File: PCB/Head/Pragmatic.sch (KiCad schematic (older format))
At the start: 11 parts, among them J1 Conn_02x07_Odd_Even, J2 Conn_02x07_Odd_Even, SW1 SW_Push, SW2 SW_Push, SW3 SW_Push, SW4 SW_Push, U1 ProMicro

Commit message: left ready
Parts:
- removed D1, D2, D3, D4: D, Foostan:D3_SMD_v2, symbol Device:D
- removed SW1, SW2, SW3, SW4: SW_Push, Foostan:CherryMX_ChocV2_1u, symbol Switch:SW_Push
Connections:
- wire segments 14 -> 0
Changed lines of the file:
@@
 Comment4 ""
 $EndDescr
-Text GLabel 1400 2100 0    50   Input ~ 0
-Row1
-Text GLabel 1400 2650 0    50   Input ~ 0
-Row2
-Text GLabel 2100 1550 1    50   Input ~ 0
-Col1
-Text GLabel 2600 1550 1    50   Input ~ 0
-Col2
-$Comp
-L Device:D D1
-U 1 1 618785C9
-P 1700 1950
-F 0 "D1" V 1700 1870 50  0000 R CNN
-F 1 "D" H 1700 2076 50  0001 C CNN
-F 2 "Foostan:D3_SMD_v2" H 1700 1950 50  0001 C CNN
-F 3 "~" H 1700 1950 50  0001 C CNN
-	1    1700 1950
-	0    -1   -1   0
-$EndComp
-Wire Wire Line
-	1400 2100 1700 2100
-Wire Wire Line
-	1400 2650 1700 2650
-$Comp
-L Switch:SW_Push SW1
-U 1 1 6187A774
-P 1900 1800
-F 0 "SW1" H 1900 1993 50  0000 C CNN
-F 1 "SW_Push" H 1900 1994 50  0001 C CNN
-F 2 "Foostan:CherryMX_ChocV2_1u" H 1900 2000 50  0001 C CNN
-F 3 "~" H 1900 2000 50  0001 C CNN
-	1    1900 1800
-	1    0    0    -1
-$EndComp
-Connection ~ 1700 2100
-Wire Wire Line
-	1700 2100 2200 2100
-$Comp
-L Device:D D3
-U 1 1 618803D0
-P 1700 2500
-F 0 "D3" V 1700 2420 50  0000 R CNN
-F 1 "D" H 1700 2626 50  0001 C CNN
-F 2 "Foostan:D3_SMD_v2" H 1700 2500 50  0001 C CNN
-F 3 "~" H 1700 2500 50  0001 C CNN
-	1    1700 2500
-	0    -1   -1   0
-$EndComp
-$Comp
-L Switch:SW_Push SW3
-U 1 1 618803DA
-P 1900 2350
-F 0 "SW3" H 1900 2543 50  0000 C CNN
-F 1 "SW_Push" H 1900 2544 50  0001 C CNN
-F 2 "Foostan:CherryMX_ChocV2_1u" H 1900 2550 50  0001 C CNN
-F 3 "~" H 1900 2550 50  0001 C CNN
-	1    1900 2350
-	1    0    0    -1
-$EndComp
-Connection ~ 2100 2350
-Wire Wire Line
-	2100 2350 2100 2650
-Wire Wire Line
-	2100 1550 2100 1800
-Wire Wire Line
-	2100 1800 2100 2350
-Connection ~ 2100 1800
-$Comp
-L Device:D D2
-U 1 1 6188DF74
-P 2200 1950
-F 0 "D2" V 2200 1870 50  0000 R CNN
-F 1 "D" H 2200 2076 50  0001 C CNN
-F 2 "Foostan:D3_SMD_v2" H 2200 1950 50  0001 C CNN
-F 3 "~" H 2200 1950 50  0001 C CNN
-	1    2200 1950
-	0    -1   -1   0
-$EndComp
-$Comp
-L Switch:SW_Push SW2
-U 1 1 6188DF7C
-P 2400 1800
-F 0 "SW2" H 2400 1993 50  0000 C CNN
-F 1 "SW_Push" H 2400 1994 50  0001 C CNN
-F 2 "Foostan:CherryMX_ChocV2_1u" H 2400 2000 50  0001 C CNN
-F 3 "~" H 2400 2000 50  0001 C CNN
-	1    2400 1800
-	1    0    0    -1
-$EndComp
-Connection ~ 2200 2100
-Wire Wire Line
-	2200 2100 2700 2100
-$Comp
-L Device:D D4
-U 1 1 6188DF84
-P 2200 2500
-F 0 "D4" V 2200 2420 50  0000 R CNN
-F 1 "D" H 2200 2626 50  0001 C CNN
-F 2 "Foostan:D3_SMD_v2" H 2200 2500 50  0001 C CNN
-F 3 "~" H 2200 2500 50  0001 C CNN
-	1    2200 2500
-	0    -1   -1   0
-$EndComp
-$Comp
-L Switch:SW_Push SW4
-U 1 1 6188DF8A
-P 2400 2350
-F 0 "SW4" H 2400 2543 50  0000 C CNN
-F 1 "SW_Push" H 2400 2544 50  0001 C CNN
-F 2 "Foostan:CherryMX_ChocV2_1u" H 2400 2550 50  0001 C CNN
-F 3 "~" H 2400 2550 50  0001 C CNN
-	1    2400 2350
-	1    0    0    -1
-$EndComp
-Connection ~ 2600 2350
-Wire Wire Line
-	2600 2350 2600 2650
-Wire Wire Line
-	2600 1550 2600 1800
-Wire Wire Line
-	2600 1800 2600 2350
-Connection ~ 2600 1800
-Wire Wire Line
-	2200 2650 2600 2650
-Connection ~ 1700 2650
-Connection ~ 2200 2650
-Wire Wire Line
-	1700 2650 2100 2650
 Text GLabel 4800 3800 0    50   Input ~ 0
 Row2
@@
 Text GLabel 6200 3600 2    50   Input ~ 0
 VCC
-Text GLabel 6600 3350 3    50   Input ~ 0
-VCC
-$Comp
-L power:+5V #PWR0101
-U 1 1 6186CA9E
-P 6600 3350
-F 0 "#PWR0101" H 6600 3200 50  0001 C CNN
-F 1 "+5V" H 6615 3523 50  0000 C CNN
-F 2 "" H 6600 3350 50  0001 C CNN
-F 3 "" H 6600 3350 50  0001 C CNN
-	1    6600 3350
-	1    0    0    -1
-$EndComp
 Text GLabel 7000 3650 0    50   Input ~ 0
 VCC
@@
 Text GLabel 4100 3650 2    50   Input ~ 0
 Ground
-Text GLabel 4100 3850 2    50   Input ~ 0
+Text GLabel 3600 4050 0    50   Input ~ 0
 Col1
-Text GLabel 4100 3950 2    50   Input ~ 0
+Text GLabel 4100 4050 2    50   Input ~ 0
 Col2
 Text GLabel 4800 3700 0    50   Input ~ 0
@@
 Text GLabel 4800 4100 0    50   Input ~ 0
 Col5
+Text GLabel 4100 4250 2    50   Input ~ 0
+Col6
 Text GLabel 3600 4250 0    50   Input ~ 0
-Col6
-Text GLabel 4100 4250 2    50   Input ~ 0
 Col5
 Text GLabel 4100 4150 2    50   Input ~ 0
@@
 Text GLabel 4800 3900 0    50   Input ~ 0
 Col3
-Text GLabel 4100 4050 2    50   Input ~ 0
+Text GLabel 3600 4150 0    50   Input ~ 0
 Col3
-Text GLabel 3600 4150 0    50   Input ~ 0
+Text GLabel 4100 3850 2    50   Input ~ 0
 Row4
-Text GLabel 3600 4050 0    50   Input ~ 0
+Text GLabel 3600 3950 0    50   Input ~ 0
 Row5
-Text GLabel 3600 3950 0    50   Input ~ 0
+Text GLabel 4100 3950 2    50   Input ~ 0
 Row6
 $Comp
@@
 	1    0    0    -1
 $EndComp
-Connection ~ 2100 2650
-Wire Wire Line
-	2100 2650 2200 2650
-Connection ~ 2600 2650
-Wire Wire Line
-	2600 2650 2700 2650
+$Comp
+L power:+5V #PWR0101
+U 1 1 6186CA9E
+P 6600 3350
+F 0 "#PWR0101" H 6600 3200 50  0001 C CNN
+F 1 "+5V" H 6615 3523 50  0000 C CNN
+F 2 "" H 6600 3350 50  0001 C CNN
+F 3 "" H 6600 3350 50  0001 C CNN
+	1    6600 3350
+	1    0    0    -1
+$EndComp
+Text GLabel 6600 3350 3    50   Input ~ 0
+VCC
 $EndSCHEMATC

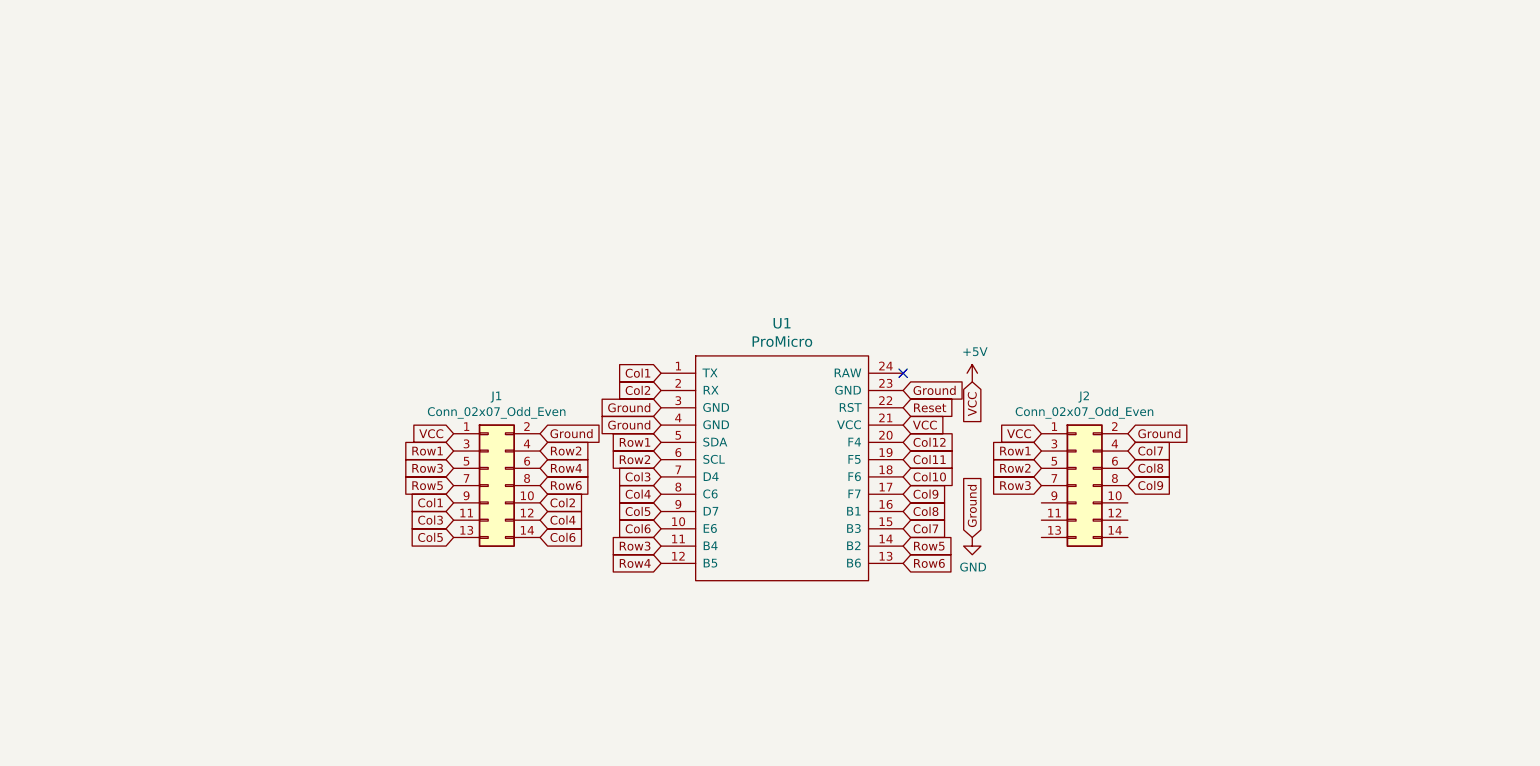
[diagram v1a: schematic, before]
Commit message: head board
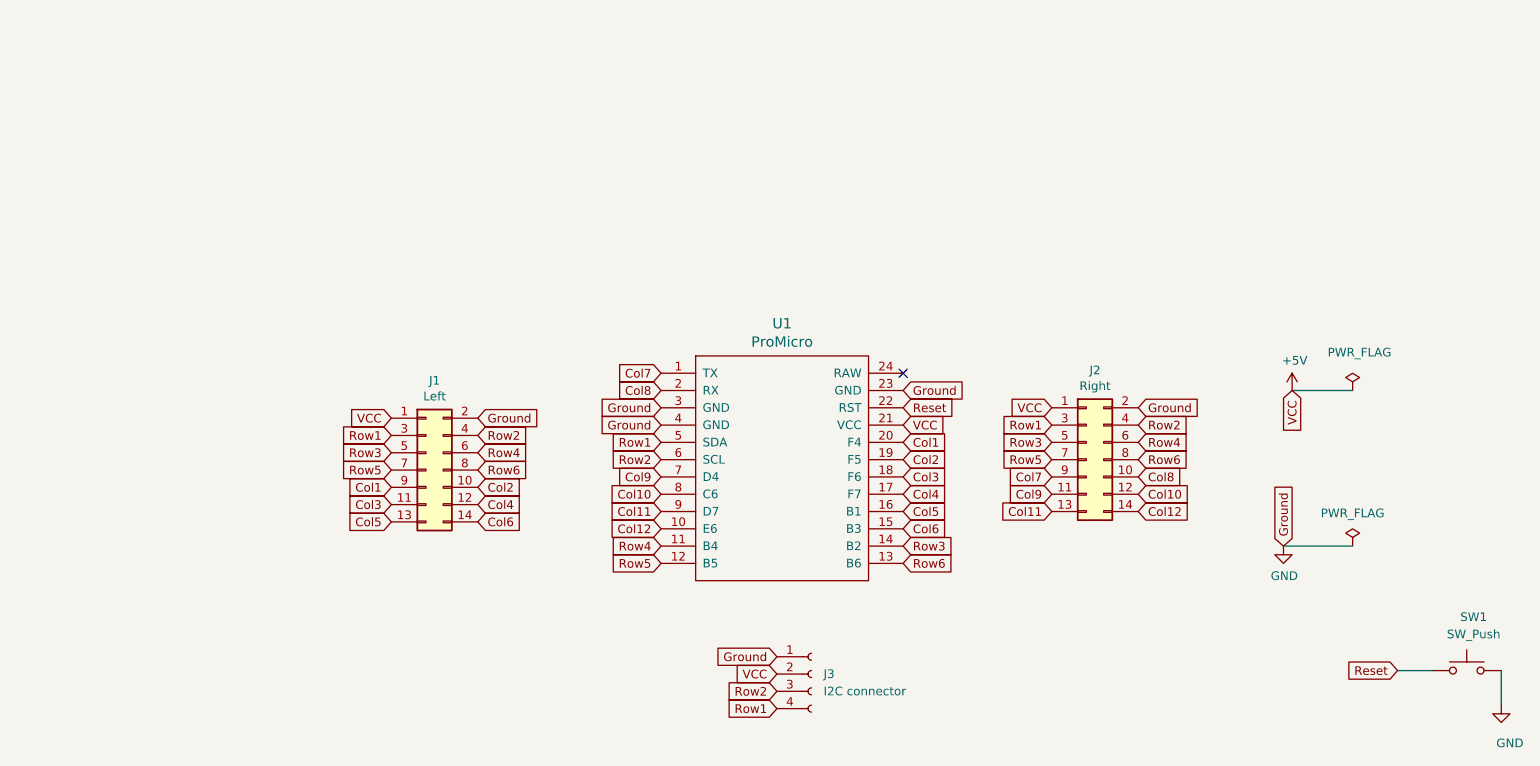
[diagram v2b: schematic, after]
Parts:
- added J3: I2C connector, Foostan:OLED_1side, symbol Connector:Conn_01x04_Female
- added SW1: SW_Push, Button_Switch_THT:SW_PUSH_6mm, symbol Switch:SW_Push
- J1: value Conn_02x07_Odd_Even -> Left
- J2: value Conn_02x07_Odd_Even -> Right
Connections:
- net +5V: now also J3.2 (Pin_2)
- net Col1: now also U1.20 (F4); no longer U1.1 (TX)
- net Col10: now also J2.12 (Pin_12), U1.8 (C6); no longer U1.18 (F6)
- net Col11: now also J2.13 (Pin_13), U1.9 (D7); no longer U1.19 (F5)
- net Col12: now also J2.14 (Pin_14), U1.10 (E6); no longer U1.20 (F4)
- net Col2: now also U1.19 (F5); no longer U1.2 (RX)
- net Col3: now also U1.18 (F6); no longer U1.7 (D4)
- net Col4: now also U1.17 (F7); no longer U1.8 (C6)
- net Col5: now also U1.16 (B1); no longer U1.9 (D7)
- net Col6: now also U1.15 (B3); no longer U1.10 (E6)
- net Col7: now also J2.9 (Pin_9), U1.1 (TX); no longer J2.4 (Pin_4), U1.15 (B3)
- net Col8: now also J2.10 (Pin_10), U1.2 (RX); no longer J2.6 (Pin_6), U1.16 (B1)
- net Col9: now also J2.11 (Pin_11), U1.7 (D4); no longer J2.8 (Pin_8), U1.17 (F7)
- net GND: now also J3.1 (Pin_1), SW1.2
- net Reset: now also SW1.1
- net Row1: now also J3.4 (Pin_4)
- net Row2: now also J2.4 (Pin_4), J3.3 (Pin_3); no longer J2.5 (Pin_5)
- net Row3: now also J2.5 (Pin_5), U1.14 (B2); no longer J2.7 (Pin_7), U1.11 (B4)
- net Row4: now also J2.6 (Pin_6), U1.11 (B4); no longer U1.12 (B5)
- net Row5: now also J2.7 (Pin_7), U1.12 (B5); no longer U1.14 (B2)
- net Row6: now also J2.8 (Pin_8)
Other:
- moved on the sheet: J1, J2
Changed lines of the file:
@@
 Text GLabel 4800 3800 0    50   Input ~ 0
 Row2
-Text GLabel 4800 3300 0    50   Input ~ 0
+Text GLabel 6200 3700 2    50   Input ~ 0
 Col1
-Text GLabel 4800 3400 0    50   Input ~ 0
+Text GLabel 6200 3800 2    50   Input ~ 0
 Col2
+Text GLabel 6200 4300 2    50   Input ~ 0
+Row3
 Text GLabel 4800 4300 0    50   Input ~ 0
-Row3
+Row4
 Text GLabel 4800 4400 0    50   Input ~ 0
-Row4
-Text GLabel 6200 4300 2    50   Input ~ 0
 Row5
 Text GLabel 6200 4400 2    50   Input ~ 0
 Row6
-Text GLabel 6200 4200 2    50   Input ~ 0
+Text GLabel 4800 3300 0    50   Input ~ 0
 Col7
-Text GLabel 6200 4100 2    50   Input ~ 0
+Text GLabel 4800 3400 0    50   Input ~ 0
 Col8
-Text GLabel 6200 4000 2    50   Input ~ 0
+Text GLabel 4800 3900 0    50   Input ~ 0
 Col9
-Text GLabel 6200 3900 2    50   Input ~ 0
+Text GLabel 4800 4000 0    50   Input ~ 0
 Col10
-Text GLabel 6200 3800 2    50   Input ~ 0
+Text GLabel 4800 4100 0    50   Input ~ 0
 Col11
-Text GLabel 6200 3700 2    50   Input ~ 0
+Text GLabel 4800 4200 0    50   Input ~ 0
 Col12
 Text GLabel 6200 3500 2    50   Input ~ 0
 Reset
-$Comp
-L power:GND #PWR0103
-U 1 1 61895032
-P 6600 4250
-F 0 "#PWR0103" H 6600 4000 50  0001 C CNN
-F 1 "GND" H 6605 4077 50  0000 C CNN
-F 2 "" H 6600 4250 50  0001 C CNN
-F 3 "" H 6600 4250 50  0001 C CNN
-	1    6600 4250
-	1    0    0    -1
-$EndComp
 NoConn ~ 6200 3300
 $Comp
 L Connector_Generic:Conn_02x07_Odd_Even J1
 U 1 1 61867C1C
-P 3800 3950
-F 0 "J1" H 3850 4467 50  0000 C CNN
-F 1 "Conn_02x07_Odd_Even" H 3850 4376 50  0000 C CNN
-F 2 "Connector_IDC:IDC-Header_2x07_P2.54mm_Vertical" H 3800 3950 50  0001 C CNN
-F 3 "~" H 3800 3950 50  0001 C CNN
-	1    3800 3950
+P 3440 3860
+F 0 "J1" H 3490 4377 50  0000 C CNN
+F 1 "Left" H 3490 4286 50  0000 C CNN
+F 2 "Connector_IDC:IDC-Header_2x07_P2.54mm_Vertical" H 3440 3860 50  0001 C CNN
+F 3 "~" H 3440 3860 50  0001 C CNN
+	1    3440 3860
 	1    0    0    -1
 $EndComp
@@
 Text GLabel 4800 3600 0    50   Input ~ 0
 Ground
-Text GLabel 6200 3400 2    50   Input ~ 0
-Ground
 Text GLabel 6200 3600 2    50   Input ~ 0
 VCC
-Text GLabel 7000 3650 0    50   Input ~ 0
-VCC
-Text GLabel 6600 4250 1    50   Input ~ 0
-Ground
-Text GLabel 7500 3650 2    50   Input ~ 0
-Ground
-Text GLabel 7000 3750 0    50   Input ~ 0
-Row1
-Text GLabel 7500 3750 2    50   Input ~ 0
-Col7
+Text GLabel 7060 3500 0    50   Input ~ 0
+VCC
+Text GLabel 7560 3500 2    50   Input ~ 0
+Ground
+Text GLabel 7060 3600 0    50   Input ~ 0
+Row1
 $Comp
 L Connector_Generic:Conn_02x07_Odd_Even J2
 U 1 1 618692F3
-P 7200 3950
-F 0 "J2" H 7250 4467 50  0000 C CNN
-F 1 "Conn_02x07_Odd_Even" H 7250 4376 50  0000 C CNN
-F 2 "Connector_IDC:IDC-Header_2x07_P2.54mm_Vertical" H 7200 3950 50  0001 C CNN
-F 3 "~" H 7200 3950 50  0001 C CNN
-	1    7200 3950
-	1    0    0    -1
-$EndComp
-Text GLabel 7500 3850 2    50   Input ~ 0
-Col8
-Text GLabel 7500 3950 2    50   Input ~ 0
-Col9
-Text GLabel 7000 3850 0    50   Input ~ 0
-Row2
-Text GLabel 7000 3950 0    50   Input ~ 0
+P 7260 3800
+F 0 "J2" H 7310 4317 50  0000 C CNN
+F 1 "Right" H 7310 4226 50  0000 C CNN
+F 2 "Connector_IDC:IDC-Header_2x07_P2.54mm_Vertical" H 7260 3800 50  0001 C CNN
+F 3 "~" H 7260 3800 50  0001 C CNN
+	1    7260 3800
+	1    0    0    -1
+$EndComp
+Text GLabel 3240 3560 0    50   Input ~ 0
+VCC
+Text GLabel 3240 3660 0    50   Input ~ 0
+Row1
+Text GLabel 3740 3660 2    50   Input ~ 0
+Row2
+Text GLabel 3240 3760 0    50   Input ~ 0
 Row3
-Text GLabel 3600 3650 0    50   Input ~ 0
-VCC
-Text GLabel 3600 3750 0    50   Input ~ 0
-Row1
-Text GLabel 4100 3750 2    50   Input ~ 0
-Row2
-Text GLabel 3600 3850 0    50   Input ~ 0
-Row3
-Text GLabel 4100 3650 2    50   Input ~ 0
-Ground
-Text GLabel 3600 4050 0    50   Input ~ 0
+Text GLabel 3740 3560 2    50   Input ~ 0
+Ground
+Text GLabel 3240 3960 0    50   Input ~ 0
 Col1
-Text GLabel 4100 4050 2    50   Input ~ 0
+Text GLabel 3740 3960 2    50   Input ~ 0
 Col2
 Text GLabel 4800 3700 0    50   Input ~ 0
 Row1
-Text GLabel 4800 4200 0    50   Input ~ 0
+Text GLabel 6200 4200 2    50   Input ~ 0
 Col6
-Text GLabel 4800 4100 0    50   Input ~ 0
+Text GLabel 6200 4100 2    50   Input ~ 0
 Col5
-Text GLabel 4100 4250 2    50   Input ~ 0
+Text GLabel 3740 4160 2    50   Input ~ 0
 Col6
-Text GLabel 3600 4250 0    50   Input ~ 0
+Text GLabel 3240 4160 0    50   Input ~ 0
 Col5
-Text GLabel 4100 4150 2    50   Input ~ 0
+Text GLabel 3740 4060 2    50   Input ~ 0
 Col4
-Text GLabel 4800 4000 0    50   Input ~ 0
+Text GLabel 6200 4000 2    50   Input ~ 0
 Col4
-Text GLabel 4800 3900 0    50   Input ~ 0
+Text GLabel 3240 4060 0    50   Input ~ 0
 Col3
-Text GLabel 3600 4150 0    50   Input ~ 0
-Col3
-Text GLabel 4100 3850 2    50   Input ~ 0
+Text GLabel 3740 3760 2    50   Input ~ 0
 Row4
-Text GLabel 3600 3950 0    50   Input ~ 0
+Text GLabel 3240 3860 0    50   Input ~ 0
 Row5
-Text GLabel 4100 3950 2    50   Input ~ 0
+Text GLabel 3740 3860 2    50   Input ~ 0
 Row6
 $Comp
@@
 	1    0    0    -1
 $EndComp
+Text GLabel 6200 3400 2    50   Input ~ 0
+Ground
+Text GLabel 7560 3600 2    50   Input ~ 0
+Row2
+Text GLabel 7060 3700 0    50   Input ~ 0
+Row3
+Text GLabel 7560 3700 2    50   Input ~ 0
+Row4
+Text GLabel 7060 3800 0    50   Input ~ 0
+Row5
+Text GLabel 7560 3800 2    50   Input ~ 0
+Row6
+Text GLabel 7060 3900 0    50   Input ~ 0
+Col7
+Text GLabel 7560 3900 2    50   Input ~ 0
+Col8
+Text GLabel 7060 4000 0    50   Input ~ 0
+Col9
+Text GLabel 7560 4000 2    50   Input ~ 0
+Col10
+Text GLabel 7060 4100 0    50   Input ~ 0
+Col11
+Text GLabel 7560 4100 2    50   Input ~ 0
+Col12
+$Comp
+L Switch:SW_Push SW1
+U 1 1 61879342
+P 9460 5020
+F 0 "SW1" H 9500 5330 50  0000 C CNN
+F 1 "SW_Push" H 9500 5230 50  0000 C CNN
+F 2 "Button_Switch_THT:SW_PUSH_6mm" H 9460 5220 50  0001 C CNN
+F 3 "~" H 9460 5220 50  0001 C CNN
+	1    9460 5020
+	1    0    0    -1
+$EndComp
+$Comp
+L power:GND #PWR01
+U 1 1 6187A59F
+P 9660 5220
+F 0 "#PWR01" H 9660 4970 50  0001 C CNN
+F 1 "GND" H 9710 5000 50  0000 C CNN
+F 2 "" H 9660 5220 50  0001 C CNN
+F 3 "" H 9660 5220 50  0001 C CNN
+	1    9660 5220
+	1    0    0    -1
+$EndComp
+Wire Wire Line
+	9660 5020 9660 5220
+Text GLabel 9060 5020 0    50   Input ~ 0
+Reset
+Wire Wire Line
+	9060 5020 9260 5020
+Text GLabel 6200 3900 2    50   Input ~ 0
+Col3
+$Comp
+L power:GND #PWR0103
+U 1 1 61895032
+P 8400 4300
+F 0 "#PWR0103" H 8400 4050 50  0001 C CNN
+F 1 "GND" H 8405 4127 50  0000 C CNN
+F 2 "" H 8400 4300 50  0001 C CNN
+F 3 "" H 8400 4300 50  0001 C CNN
+	1    8400 4300
+	1    0    0    -1
+$EndComp
+Text GLabel 8400 4300 1    50   Input ~ 0
+Ground
 $Comp
 L power:+5V #PWR0101
 U 1 1 6186CA9E
-P 6600 3350
-F 0 "#PWR0101" H 6600 3200 50  0001 C CNN
-F 1 "+5V" H 6615 3523 50  0000 C CNN
-F 2 "" H 6600 3350 50  0001 C CNN
-F 3 "" H 6600 3350 50  0001 C CNN
-	1    6600 3350
-	1    0    0    -1
-$EndComp
-Text GLabel 6600 3350 3    50   Input ~ 0
-VCC
+P 8450 3400
+F 0 "#PWR0101" H 8450 3250 50  0001 C CNN
+F 1 "+5V" H 8465 3573 50  0000 C CNN
+F 2 "" H 8450 3400 50  0001 C CNN
+F 3 "" H 8450 3400 50  0001 C CNN
+	1    8450 3400
+	1    0    0    -1
+$EndComp
+Text GLabel 8450 3400 3    50   Input ~ 0
+VCC
+$Comp
+L power:PWR_FLAG #FLG0101
+U 1 1 61894CD0
+P 8800 3400
+F 0 "#FLG0101" H 8800 3475 50  0001 C CNN
+F 1 "PWR_FLAG" H 8840 3620 50  0000 C CNN
+F 2 "" H 8800 3400 50  0001 C CNN
+F 3 "~" H 8800 3400 50  0001 C CNN
+	1    8800 3400
+	1    0    0    -1
+$EndComp
+Wire Wire Line
+	8800 3400 8450 3400
+$Comp
+L power:PWR_FLAG #FLG0102
+U 1 1 6189758B
+P 8800 4300
+F 0 "#FLG0102" H 8800 4375 50  0001 C CNN
+F 1 "PWR_FLAG" H 8800 4490 50  0000 C CNN
+F 2 "" H 8800 4300 50  0001 C CNN
+F 3 "~" H 8800 4300 50  0001 C CNN
+	1    8800 4300
+	1    0    0    -1
+$EndComp
+Wire Wire Line
+	8400 4300 8800 4300
+$Comp
+L Connector:Conn_01x04_Female J3
+U 1 1 618A512B
+P 5670 5040
+F 0 "J3" H 5740 5040 50  0000 L CNN
+F 1 "I2C connector" H 5740 4940 50  0000 L CNN
+F 2 "Foostan:OLED_1side" H 5670 5040 50  0001 C CNN
+F 3 "~" H 5670 5040 50  0001 C CNN
+	1    5670 5040
+	1    0    0    -1
+$EndComp
+Text GLabel 5470 5040 0    50   Input ~ 0
+VCC
+Text GLabel 5470 5140 0    50   Input ~ 0
+Row2
+Text GLabel 5470 5240 0    50   Input ~ 0
+Row1
+Text GLabel 5470 4940 0    50   Input ~ 0
+Ground
 $EndSCHEMATC

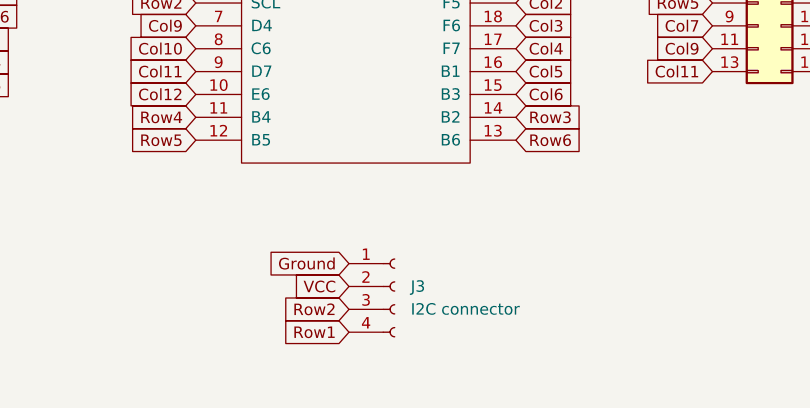
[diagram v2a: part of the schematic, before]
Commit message: finish up
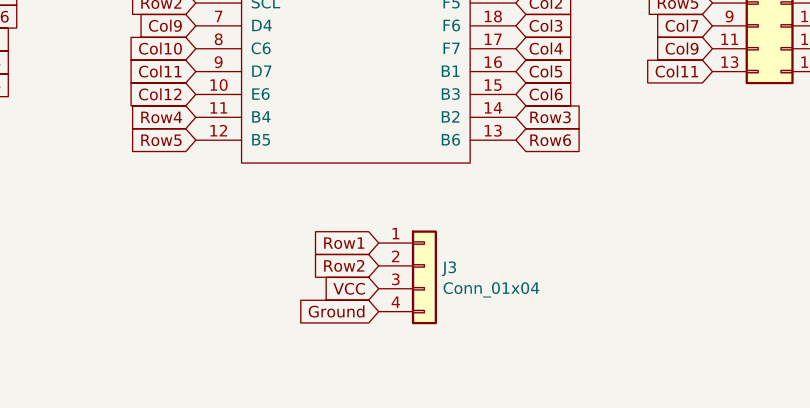
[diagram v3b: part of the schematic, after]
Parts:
- removed J3: I2C connector, Foostan:OLED_1side, symbol Connector:Conn_01x04_Female
- added J3: Conn_01x04, Connector_PinSocket_2.54mm:PinSocket_1x04_P2.54mm_Vertical, symbol Connector_Generic:Conn_01x04
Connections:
- net +5V: now also J3.3 (Pin_3)
- net GND: now also J3.4 (Pin_4)
- net Row1: now also J3.1 (Pin_1)
- net Row2: now also J3.2 (Pin_2)
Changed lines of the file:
@@
 	8400 4300 8800 4300
 $Comp
-L Connector:Conn_01x04_Female J3
-U 1 1 618A512B
-P 5670 5040
-F 0 "J3" H 5740 5040 50  0000 L CNN
-F 1 "I2C connector" H 5740 4940 50  0000 L CNN
-F 2 "Foostan:OLED_1side" H 5670 5040 50  0001 C CNN
-F 3 "~" H 5670 5040 50  0001 C CNN
-	1    5670 5040
+L Connector_Generic:Conn_01x04 J3
+U 1 1 6189149E
+P 5800 4950
+F 0 "J3" H 5880 4942 50  0000 L CNN
+F 1 "Conn_01x04" H 5880 4851 50  0000 L CNN
+F 2 "Connector_PinSocket_2.54mm:PinSocket_1x04_P2.54mm_Vertical" H 5800 4950 50  0001 C CNN
+F 3 "~" H 5800 4950 50  0001 C CNN
+	1    5800 4950
 	1    0    0    -1
 $EndComp
-Text GLabel 5470 5040 0    50   Input ~ 0
+Text GLabel 5600 5050 0    50   Input ~ 0
 VCC
-Text GLabel 5470 5140 0    50   Input ~ 0
+Text GLabel 5600 5150 0    50   Input ~ 0
+Ground
+Text GLabel 5600 4950 0    50   Input ~ 0
 Row2
-Text GLabel 5470 5240 0    50   Input ~ 0
+Text GLabel 5600 4850 0    50   Input ~ 0
 Row1
-Text GLabel 5470 4940 0    50   Input ~ 0
-Ground
 $EndSCHEMATC
